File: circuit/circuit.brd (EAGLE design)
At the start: 100 x 80 mm, 60 parts, among them IC1 74HC04N, X1 PSS 254/8G

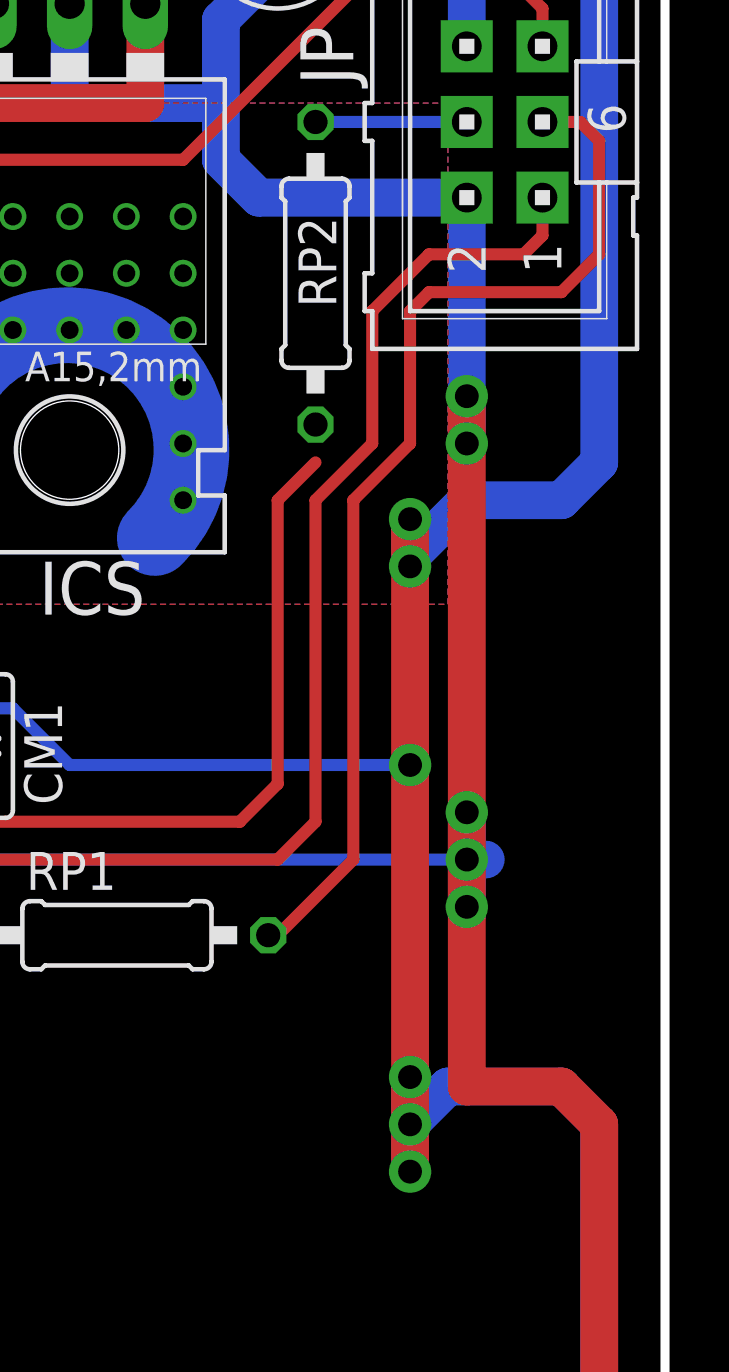
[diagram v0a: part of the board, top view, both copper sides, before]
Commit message: minor changes
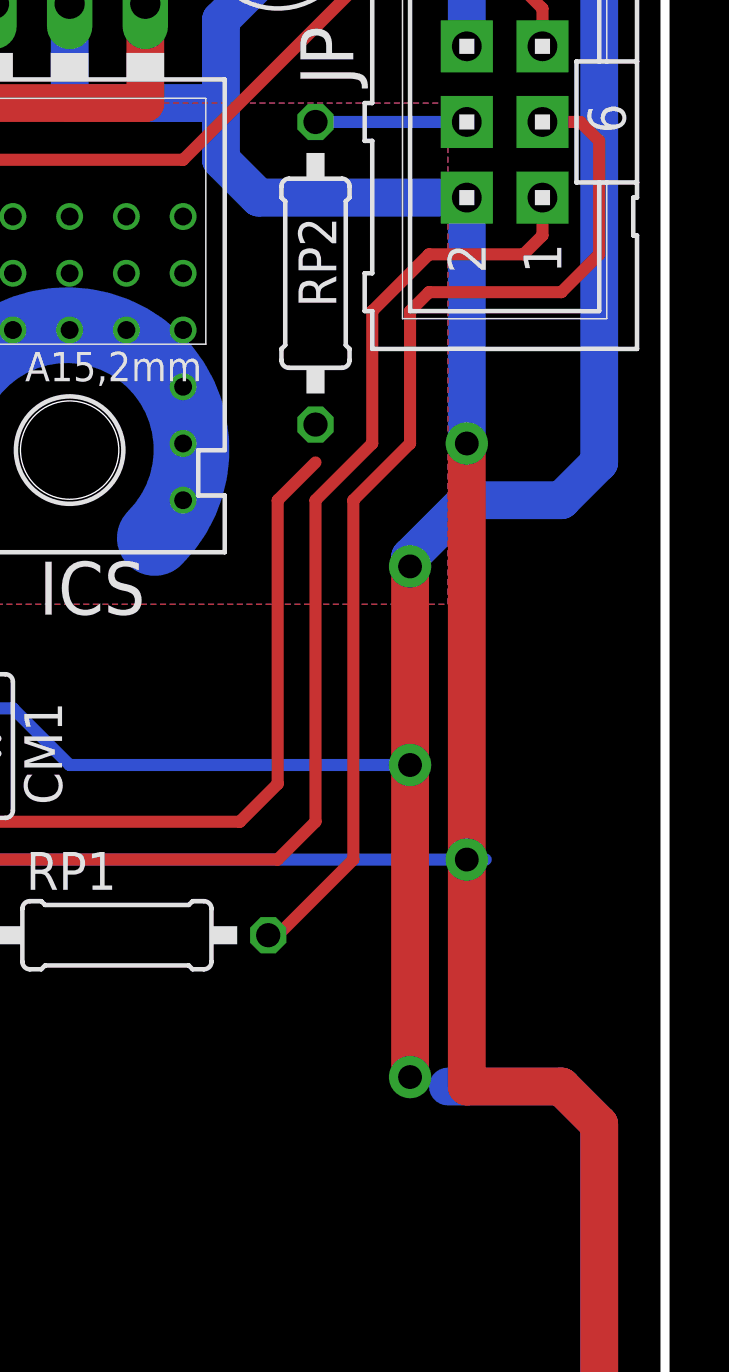
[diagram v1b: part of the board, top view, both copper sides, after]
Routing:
- net GND: track 542.0 -> 531.0 mm, vias 6 -> 3
- net +5V: track 432.8 -> 427.0 mm, vias 7 -> 4
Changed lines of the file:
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@@
 <wire x1="85.09" y1="64.389" x2="86.995" y2="66.294" width="1.27" layer="16"/>
 <via x="93.345" y="36.195" extent="1-16" drill="0.8" diameter="1.4224"/>
-<wire x1="93.345" y1="36.195" x2="93.98" y2="36.195" width="1.27" layer="16"/>
+<wire x1="93.345" y1="36.195" x2="93.98" y2="36.195" width="0" layer="19" extent="1-16"/>
 <wire x1="97.79" y1="27.305" x2="96.52" y2="28.575" width="1.27" layer="1"/>
-<wire x1="93.345" y1="28.575" x2="93.345" y2="34.6075" width="1.27" layer="1"/>
-<wire x1="93.345" y1="34.6075" x2="93.345" y2="36.195" width="1.27" layer="1"/>
+<wire x1="93.345" y1="28.575" x2="93.345" y2="36.195" width="1.27" layer="1"/>
+<wire x1="93.345" y1="34.6075" x2="93.345" y2="36.195" width="0" layer="19" extent="1-16"/>
 <wire x1="96.52" y1="28.575" x2="93.345" y2="28.575" width="1.27" layer="1"/>
-<wire x1="93.345" y1="36.195" x2="93.345" y2="37.7825" width="1.27" layer="1"/>
+<wire x1="93.345" y1="36.195" x2="93.345" y2="37.7825" width="0" layer="19" extent="1-16"/>
 <via x="93.345" y="50.165" extent="1-16" drill="0.8" diameter="1.4224"/>
-<wire x1="93.345" y1="37.7825" x2="93.345" y2="50.165" width="1.27" layer="1"/>
-<wire x1="93.345" y1="50.165" x2="93.345" y2="51.7525" width="1.27" layer="16"/>
-<via x="93.345" y="34.6075" extent="1-16" drill="0.8" diameter="1.4224"/>
-<via x="93.345" y="37.7825" extent="1-16" drill="0.8" diameter="1.4224"/>
-<wire x1="93.345" y1="51.7525" x2="93.345" y2="58.42" width="1.27" layer="16"/>
-<wire x1="93.345" y1="37.7825" x2="93.345" y2="34.6075" width="1.27" layer="16"/>
-<via x="93.345" y="51.7525" extent="1-16" drill="0.8" diameter="1.4224"/>
-<wire x1="93.345" y1="34.29" x2="93.345" y2="34.6075" width="1.27" layer="16"/>
-<wire x1="93.345" y1="51.7525" x2="93.345" y2="50.165" width="1.27" layer="1"/>
+<wire x1="93.345" y1="36.195" x2="93.345" y2="50.165" width="1.27" layer="1"/>
+<wire x1="93.345" y1="50.165" x2="93.345" y2="51.7525" width="0" layer="19" extent="1-16"/>
+<wire x1="93.345" y1="34.6075" x2="93.345" y2="34.6075" width="0" layer="19" extent="1-16"/>
+<wire x1="93.345" y1="37.7825" x2="93.345" y2="37.7825" width="0" layer="19" extent="1-16"/>
+<wire x1="93.345" y1="50.165" x2="93.345" y2="58.42" width="1.27" layer="16"/>
+<wire x1="93.345" y1="37.7825" x2="93.345" y2="34.29" width="0" layer="19" extent="1-16"/>
+<wire x1="93.345" y1="51.7525" x2="93.345" y2="51.7525" width="0" layer="19" extent="1-16"/>
+<wire x1="93.345" y1="34.29" x2="93.345" y2="34.6075" width="0" layer="19" extent="1-16"/>
+<wire x1="93.345" y1="51.7525" x2="93.345" y2="50.165" width="0" layer="19" extent="1-16"/>
 <wire x1="58.42" y1="43.815" x2="60.96" y2="41.275" width="0.4064" layer="16"/>
 <wire x1="60.96" y1="41.275" x2="62.23" y2="41.275" width="0.4064" layer="16"/>
@@
 <wire x1="73.66" y1="66.675" x2="73.66" y2="66.04" width="0.3048" layer="1"/>
 <wire x1="1.905" y1="11.43" x2="1.905" y2="64.135" width="1.27" layer="16"/>
-<wire x1="91.44" y1="25.7175" x2="91.44" y2="27.305" width="1.27" layer="1"/>
-<wire x1="91.44" y1="27.305" x2="92.71" y2="28.575" width="1.27" layer="16"/>
+<wire x1="91.44" y1="25.7175" x2="91.44" y2="27.305" width="0" layer="19" extent="1-16"/>
+<wire x1="91.44" y1="27.305" x2="92.71" y2="28.575" width="0" layer="19" extent="1-16"/>
 <wire x1="92.71" y1="28.575" x2="96.52" y2="28.575" width="1.27" layer="16"/>
-<via x="91.44" y="27.305" extent="1-16" drill="0.8" diameter="1.4224"/>
+<wire x1="91.44" y1="27.305" x2="91.44" y2="27.305" width="0" layer="19" extent="1-16"/>
 <wire x1="93.345" y1="63.5" x2="93.345" y2="68.58" width="1.27" layer="16"/>
 <wire x1="93.345" y1="68.58" x2="86.995" y2="68.58" width="1.27" layer="16"/>
@@
 <wire x1="86.995" y1="68.326" x2="86.995" y2="68.58" width="1.27" layer="16"/>
 <wire x1="85.725" y1="74.93" x2="85.725" y2="68.58" width="1.27" layer="16"/>
-<via x="91.44" y="25.7175" extent="1-16" drill="0.8" diameter="1.4224"/>
-<wire x1="91.44" y1="27.305" x2="91.44" y2="25.7175" width="1.27" layer="16"/>
+<wire x1="91.44" y1="25.7175" x2="91.44" y2="25.7175" width="0" layer="19" extent="1-16"/>
+<wire x1="91.44" y1="27.305" x2="91.44" y2="25.7175" width="0" layer="19" extent="1-16"/>
 <wire x1="97.79" y1="49.53" x2="96.52" y2="48.26" width="1.27" layer="16"/>
 <wire x1="96.52" y1="48.26" x2="93.345" y2="48.26" width="1.27" layer="16"/>
-<wire x1="91.44" y1="47.625" x2="91.44" y2="46.0375" width="1.27" layer="1"/>
-<via x="91.44" y="47.625" extent="1-16" drill="0.8" diameter="1.4224"/>
+<wire x1="91.44" y1="47.625" x2="91.44" y2="46.0375" width="0" layer="19" extent="1-16"/>
+<wire x1="91.44" y1="47.625" x2="91.44" y2="47.625" width="0" layer="19" extent="1-16"/>
 <wire x1="91.44" y1="46.0375" x2="91.44" y2="39.37" width="1.27" layer="1"/>
 <wire x1="91.44" y1="39.37" x2="91.44" y2="28.8925" width="1.27" layer="1"/>
-<wire x1="91.44" y1="28.8925" x2="91.44" y2="27.305" width="1.27" layer="1"/>
+<wire x1="91.44" y1="28.8925" x2="91.44" y2="27.305" width="0" layer="19" extent="1-16"/>
 <via x="91.44" y="28.8925" extent="1-16" drill="0.8" diameter="1.4224"/>
-<wire x1="91.44" y1="28.8925" x2="91.44" y2="27.305" width="1.27" layer="16"/>
+<wire x1="91.44" y1="28.8925" x2="91.44" y2="27.305" width="0" layer="19" extent="1-16"/>
 <via x="91.44" y="46.0375" extent="1-16" drill="0.8" diameter="1.4224"/>
-<wire x1="91.44" y1="46.355" x2="91.44" y2="47.625" width="1.27" layer="16"/>
+<wire x1="91.44" y1="46.355" x2="91.44" y2="47.625" width="0" layer="19" extent="1-16"/>
 <wire x1="93.345" y1="48.26" x2="91.44" y2="46.355" width="1.27" layer="16"/>
 <wire x1="91.44" y1="46.355" x2="91.44" y2="46.0375" width="1.27" layer="16"/>
